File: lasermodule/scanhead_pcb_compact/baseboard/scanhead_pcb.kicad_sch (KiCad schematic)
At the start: 5 parts, among them J1 Connector_Generic_Conn_01x02, J2 FPC 15 pin molex vertical, U10 MCP1700x-330xxTT, U9 LM7805_TO220

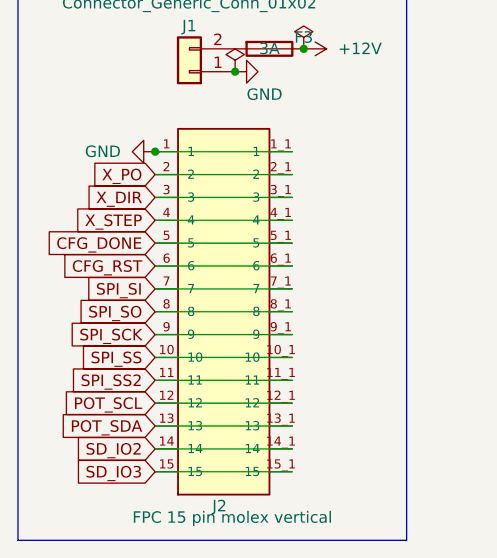
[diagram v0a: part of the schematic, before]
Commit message: laid out board
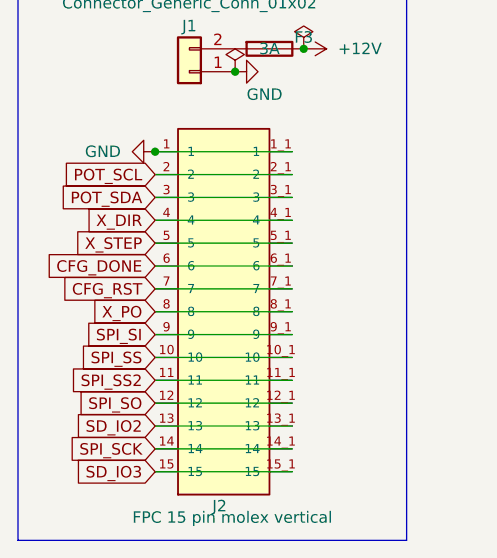
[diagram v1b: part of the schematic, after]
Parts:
- J1: footprint Connector_AMASS:AMASS_XT60-F_1x02_P7.20mm_Vertical -> Connector_AMASS:AMASS_XT30PW-F_1x02_P2.50mm_Horizontal
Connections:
- net CFG_DONE: now also J2.6, J2.6_1 (6); no longer J2.5, J2.5_1 (5)
- net CFG_RST: now also J2.7, J2.7_1 (7); no longer J2.6, J2.6_1 (6)
- net POT_SCL: now also J2.2, J2.2_1 (2); no longer J2.12, J2.12_1 (12)
- net POT_SDA: now also J2.3, J2.3_1 (3); no longer J2.13, J2.13_1 (13)
- net SD_IO2: now also J2.13, J2.13_1 (13); no longer J2.14, J2.14_1 (14)
- net SPI_SCK: now also J2.14, J2.14_1 (14); no longer J2.9, J2.9_1 (9)
- net SPI_SI: now also J2.9, J2.9_1 (9); no longer J2.7, J2.7_1 (7)
- net SPI_SO: now also J2.12, J2.12_1 (12); no longer J2.8, J2.8_1 (8)
- net X_DIR: now also J2.4, J2.4_1 (4); no longer J2.3, J2.3_1 (3)
- net X_PO: now also J2.8, J2.8_1 (8); no longer J2.2, J2.2_1 (2)
- net X_STEP: now also J2.5, J2.5_1 (5); no longer J2.4, J2.4_1 (4)
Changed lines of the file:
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@@
     (effects (font (size 3 3)) (justify left bottom))
   )
-  (global_label "SPI_SI" (shape input) (at 52.07 86.36 180) (fields_autoplaced)
-    (effects (font (size 1.27 1.27)) (justify right))
-    (property "Intersheetrefs" "${INTERSHEET_REFS}" (at 43.8796 86.2806 0)
-      (effects (font (size 1.27 1.27)) (justify right) hide)
-    )
-  )
-  (global_label "X_DIR" (shape input) (at 52.07 76.2 180) (fields_autoplaced)
-    (effects (font (size 1.27 1.27)) (justify right))
-    (property "Intersheetrefs" "${INTERSHEET_REFS}" (at -193.04 19.05 0)
+  (global_label "SPI_SI" (shape input) (at 52.07 91.44 180) (fields_autoplaced)
+    (effects (font (size 1.27 1.27)) (justify right))
+    (property "Intersheetrefs" "${INTERSHEET_REFS}" (at 43.8796 91.3606 0)
+      (effects (font (size 1.27 1.27)) (justify right) hide)
+    )
+  )
+  (global_label "X_DIR" (shape input) (at 52.07 78.74 180) (fields_autoplaced)
+    (effects (font (size 1.27 1.27)) (justify right))
+    (property "Intersheetrefs" "${INTERSHEET_REFS}" (at -193.04 21.59 0)
       (effects (font (size 1.27 1.27)) hide)
     )
@@
     )
   )
-  (global_label "CFG_RST" (shape input) (at 52.07 83.82 180) (fields_autoplaced)
-    (effects (font (size 1.27 1.27)) (justify right))
-    (property "Intersheetrefs" "${INTERSHEET_REFS}" (at 41.7025 83.7406 0)
-      (effects (font (size 1.27 1.27)) (justify right) hide)
-    )
-  )
-  (global_label "POT_SDA" (shape input) (at 52.07 101.6 180) (fields_autoplaced)
-    (effects (font (size 1.27 1.27)) (justify right))
-    (property "Intersheetrefs" "${INTERSHEET_REFS}" (at 41.642 101.5206 0)
-      (effects (font (size 1.27 1.27)) (justify right) hide)
-    )
-  )
-  (global_label "SD_IO2" (shape input) (at 52.07 104.14 180) (fields_autoplaced)
-    (effects (font (size 1.27 1.27)) (justify right))
-    (property "Intersheetrefs" "${INTERSHEET_REFS}" (at 43.1539 104.0606 0)
-      (effects (font (size 1.27 1.27)) (justify right) hide)
-    )
-  )
-  (global_label "CFG_DONE" (shape input) (at 52.07 81.28 180) (fields_autoplaced)
-    (effects (font (size 1.27 1.27)) (justify right))
-    (property "Intersheetrefs" "${INTERSHEET_REFS}" (at 40.0696 81.2006 0)
-      (effects (font (size 1.27 1.27)) (justify right) hide)
-    )
-  )
-  (global_label "X_STEP" (shape input) (at 52.07 78.74 180) (fields_autoplaced)
-    (effects (font (size 1.27 1.27)) (justify right))
-    (property "Intersheetrefs" "${INTERSHEET_REFS}" (at 42.9725 78.6606 0)
-      (effects (font (size 1.27 1.27)) (justify right) hide)
-    )
-  )
-  (global_label "SPI_SO" (shape input) (at 52.07 88.9 180) (fields_autoplaced)
-    (effects (font (size 1.27 1.27)) (justify right))
-    (property "Intersheetrefs" "${INTERSHEET_REFS}" (at 43.1539 88.8206 0)
+  (global_label "CFG_RST" (shape input) (at 52.07 86.36 180) (fields_autoplaced)
+    (effects (font (size 1.27 1.27)) (justify right))
+    (property "Intersheetrefs" "${INTERSHEET_REFS}" (at 41.7025 86.2806 0)
+      (effects (font (size 1.27 1.27)) (justify right) hide)
+    )
+  )
+  (global_label "POT_SDA" (shape input) (at 52.07 76.2 180) (fields_autoplaced)
+    (effects (font (size 1.27 1.27)) (justify right))
+    (property "Intersheetrefs" "${INTERSHEET_REFS}" (at 41.642 76.1206 0)
+      (effects (font (size 1.27 1.27)) (justify right) hide)
+    )
+  )
+  (global_label "SD_IO2" (shape input) (at 52.07 101.6 180) (fields_autoplaced)
+    (effects (font (size 1.27 1.27)) (justify right))
+    (property "Intersheetrefs" "${INTERSHEET_REFS}" (at 43.1539 101.5206 0)
+      (effects (font (size 1.27 1.27)) (justify right) hide)
+    )
+  )
+  (global_label "CFG_DONE" (shape input) (at 52.07 83.82 180) (fields_autoplaced)
+    (effects (font (size 1.27 1.27)) (justify right))
+    (property "Intersheetrefs" "${INTERSHEET_REFS}" (at 40.0696 83.7406 0)
+      (effects (font (size 1.27 1.27)) (justify right) hide)
+    )
+  )
+  (global_label "X_STEP" (shape input) (at 52.07 81.28 180) (fields_autoplaced)
+    (effects (font (size 1.27 1.27)) (justify right))
+    (property "Intersheetrefs" "${INTERSHEET_REFS}" (at 42.9725 81.2006 0)
+      (effects (font (size 1.27 1.27)) (justify right) hide)
+    )
+  )
+  (global_label "SPI_SO" (shape input) (at 52.07 99.06 180) (fields_autoplaced)
+    (effects (font (size 1.27 1.27)) (justify right))
+    (property "Intersheetrefs" "${INTERSHEET_REFS}" (at 43.1539 98.9806 0)
       (effects (font (size 1.27 1.27)) (justify right) hide)
     )
@@
     )
   )
-  (global_label "SPI_SCK" (shape input) (at 52.07 91.44 180) (fields_autoplaced)
-    (effects (font (size 1.27 1.27)) (justify right))
-    (property "Intersheetrefs" "${INTERSHEET_REFS}" (at 41.9444 91.3606 0)
-      (effects (font (size 1.27 1.27)) (justify right) hide)
-    )
-  )
-  (global_label "X_PO" (shape input) (at 52.07 73.66 180) (fields_autoplaced)
-    (effects (font (size 1.27 1.27)) (justify right))
-    (property "Intersheetrefs" "${INTERSHEET_REFS}" (at -193.04 13.97 0)
-      (effects (font (size 1.27 1.27)) hide)
-    )
-  )
-  (global_label "POT_SCL" (shape input) (at 52.07 99.06 180) (fields_autoplaced)
-    (effects (font (size 1.27 1.27)) (justify right))
-    (property "Intersheetrefs" "${INTERSHEET_REFS}" (at 19.05 45.72 0)
+  (global_label "SPI_SCK" (shape input) (at 52.07 104.14 180) (fields_autoplaced)
+    (effects (font (size 1.27 1.27)) (justify right))
+    (property "Intersheetrefs" "${INTERSHEET_REFS}" (at 41.9444 104.0606 0)
+      (effects (font (size 1.27 1.27)) (justify right) hide)
+    )
+  )
+  (global_label "X_PO" (shape input) (at 52.07 88.9 180) (fields_autoplaced)
+    (effects (font (size 1.27 1.27)) (justify right))
+    (property "Intersheetrefs" "${INTERSHEET_REFS}" (at -193.04 29.21 0)
+      (effects (font (size 1.27 1.27)) hide)
+    )
+  )
+  (global_label "POT_SCL" (shape input) (at 52.07 73.66 180) (fields_autoplaced)
+    (effects (font (size 1.27 1.27)) (justify right))
+    (property "Intersheetrefs" "${INTERSHEET_REFS}" (at 19.05 20.32 0)
       (effects (font (size 1.27 1.27)) hide)
     )
@@
       (effects (font (size 1.27 1.27)))
     )
-    (property "Footprint" "Connector_AMASS:AMASS_XT60-F_1x02_P7.20mm_Vertical" (at 55.88 62.23 0)
-      (effects (font (size 1.27 1.27)) hide)
-    )
+    (property "Footprint" "Connector_AMASS:AMASS_XT30PW-F_1x02_P2.50mm_Horizontal" (at 55.88 62.23 0)
+      (effects (font (size 1.27 1.27)) hide)
+    )
